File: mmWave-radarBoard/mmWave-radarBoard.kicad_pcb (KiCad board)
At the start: 6 copper layers, 100 x 100 mm, 276 parts, among them J101 Conn_01x03_Socket, J102 Conn_01x07_Socket, J103 Conn_01x06_Socket, J201 Conn_01x02_Socket, J203 USB4120-03-C, J401 Conn_01x03_Socket, J402 Conn_01x03_Socket, J403 Conn_01x03_Socket, J501 Conn_02x06_Odd_Even, Q201 BSS123, SW601 SW_DPST, SW602 SW_DPST, SW603 SW_SPDT, SW604 SW_DIP_x04, U201 TPS628502DRLR, U202 USBLC6-2P6, U203 TPS628502DRLR, U204 TPS2116DRL, U205 XI6432BRQAAMY, U206 TLV75533PDRV, U301 FT4232HQ, U302 93LCxxB, U401 TCAN1042HGVDRQ1, U402 TLIN1039DDFRQ1, U403 TRS3221EIDBR, U501 MX25R1635FZUIH0, U601 TS3A5018RSVR, U602 SN74LVC1G11DSFR, Y301 12MHz, Y501 40MHz

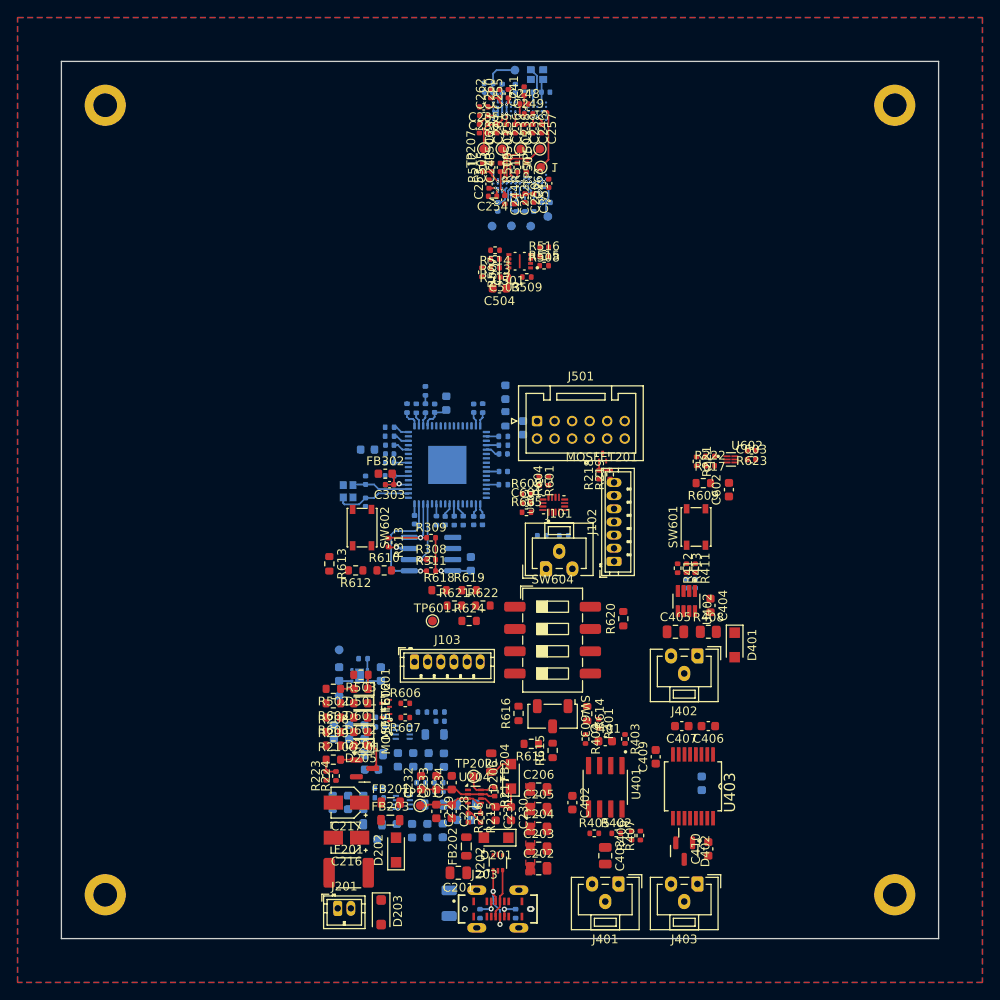
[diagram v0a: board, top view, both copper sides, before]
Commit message: Updated PCB
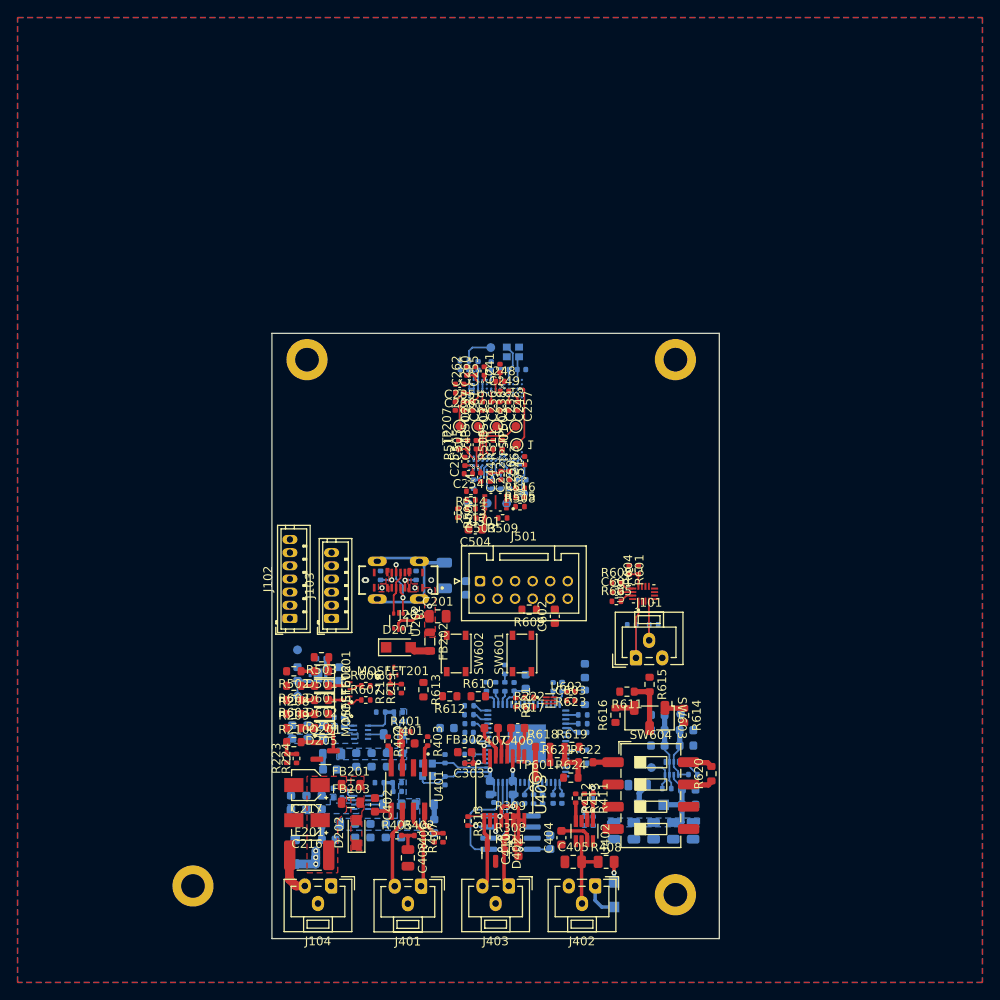
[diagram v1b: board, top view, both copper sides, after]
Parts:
- removed J201: Conn_01x02_Socket, Connector_JST:JST_ZH_B2B-ZR_1x02_P1.50mm_Vertical
- added J104: Conn_01x03_Socket, Connector_JST:JST_ZE_B03B-ZESK-D_1x03_P1.50mm_Vertical, F.Cu at (125.8, 144.0)
- C202, C203, C204, C205, C206, C228, C229, C230, C231, C232, C233, C234, C409, D203, D206, D401, FB204, R215, R216, R217, TP201, TP202, U204: moved to B.Cu
- moved R203 41.5 mm to (131.4, 108.6), turned to 90 degrees
- moved R204 39.2 mm to (135.4, 108.6), turned to 90 degrees
- moved J203 39.2 mm to (133.4, 109.1), turned to 180 degrees
- moved H102 38.3 mm to (165.0, 84.0)
- moved J102 37.5 mm to (121.0, 113.5)
- moved R207 37.4 mm to (138.7, 108.6)
- moved H101 37.0 mm to (123.0, 84.0)
- moved R617 34.3 mm to (148.3, 122.5)
- moved R623 34.3 mm to (153.1, 121.8)
- moved R221 34.3 mm to (146.8, 123.1)
- moved R222 34.3 mm to (148.3, 123.6)
- moved C603 34.3 mm to (153.1, 122.9)
- moved U602 34.3 mm to (150.7, 122.8)
- moved MOSFET201 34.1 mm to (132.9, 119.5)
- moved R218 34.1 mm to (132.5, 121.5)
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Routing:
- net Net-(J203-SHIELD-PadS1): track 0.00 -> 17.9 mm
- net VCC_3V3: track 3.19 -> 18.6 mm, vias 0 -> 1
- net /I2C_SCL: track 0.00 -> 10.4 mm
- net /COM busses/CAN_L: track 0.00 -> 9.13 mm
- net /COM busses/CAN_H: track 0.00 -> 9.13 mm
- net /COM busses/LIN: track 0.00 -> 9.01 mm
- net /COM busses/TX: track 0.00 -> 7.89 mm
- net /COM busses/RX: track 0.00 -> 7.87 mm
- net 5V_IN: track 10.3 -> 17.7 mm
- net /I2C_SDA: track 0.00 -> 6.25 mm
- net Net-(SW603-B): track 0.00 -> 5.90 mm
- net /Power/1V8_FB: track 0.00 -> 5.42 mm
- net /Power/1V2_FB: track 0.00 -> 5.17 mm
- net Net-(R619-Pad1): track 0.00 -> 5.13 mm
- net Net-(J104-Pin_3): track 0.00 -> 4.79 mm
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- added copper zone on B.Cu, net 5V_IN
- added copper zone on B.Cu, net 5V_IN_USB
- added copper zone on F.Cu, net DC_IN
- added copper zone on F.Cu, net Net-(D202-A)
- added copper zone on B.Cu, net REG_OUT_1V2
- added copper zone on B.Cu, net REG_OUT_1V8
- added copper zone on F.Cu, net USB_5V
- added copper zone on In2.Cu, net USB_5V
- removed copper zone on F.Cu, net 5V_IN_USB
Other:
- board size 100 x 100 mm -> 51 x 69 mm

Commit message: Updated schematic and layout PCB
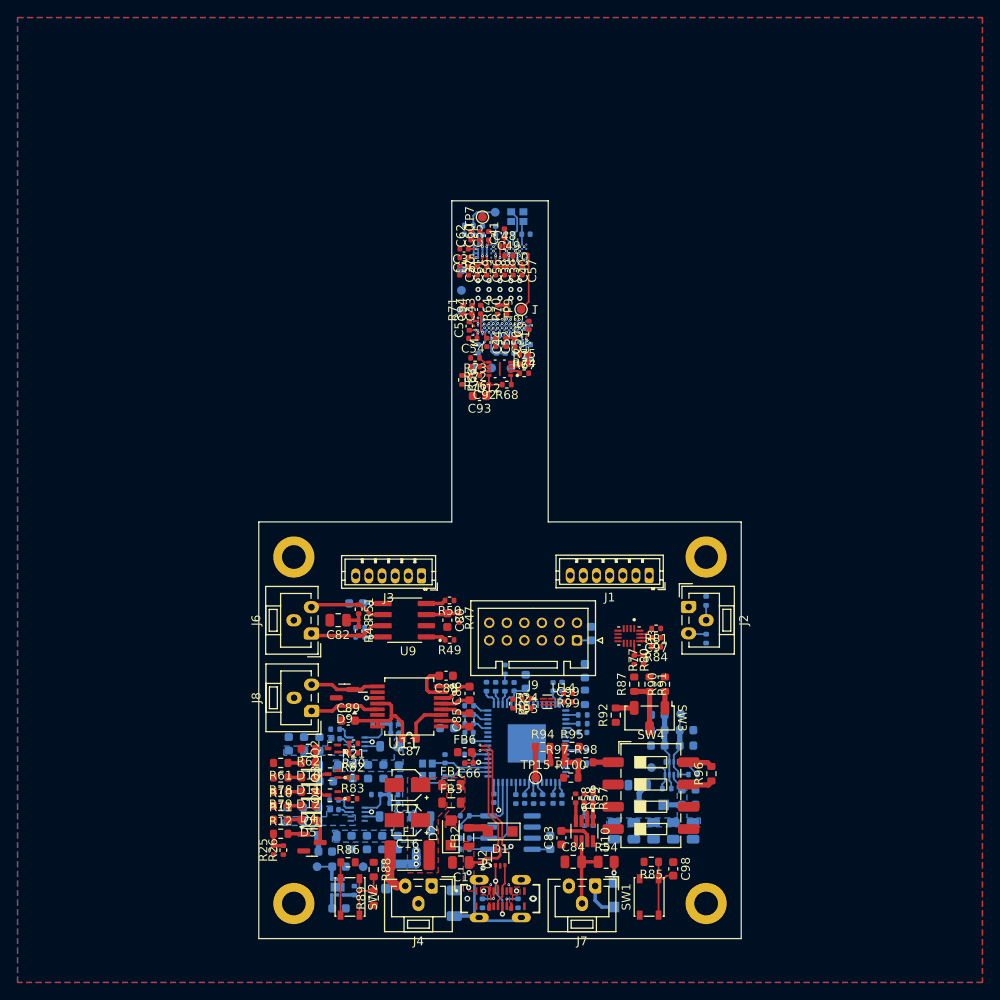
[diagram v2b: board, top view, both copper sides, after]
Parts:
- C81: renamed from C402; moved to B.Cu
- C87: renamed from C408; moved to F.Cu
- C88: renamed from C409; moved to F.Cu
- Q2: renamed from MOSFET201; footprint SSM3K35AMFV:VESM_TOS-L -> SSM3K35AMFV:VESM_TOS-M
- Q3: renamed from MOSFET601; footprint SSM3K35AMFV:VESM_TOS-L -> SSM3K35AMFV:VESM_TOS-M
- Q4: renamed from MOSFET602; footprint SSM3K35AMFV:VESM_TOS-L -> SSM3K35AMFV:VESM_TOS-M
- R35: renamed from R308; moved to B.Cu
- R36: renamed from R309; moved to B.Cu
- R38: renamed from R311; moved to B.Cu
- R40: renamed from R313; moved to B.Cu
- R52: renamed from R406; moved to B.Cu
- R53: renamed from R407; moved to B.Cu
- TP11: renamed from TP503; moved to B.Cu
- TP13: renamed from TP505; moved to B.Cu
- TP14: renamed from TP506; moved to B.Cu
- moved J1 41.2 mm to (162.0, 108.6), turned to 180 degrees
- moved R5 40.5 mm to (147.1, 146.0), turned to -90 degrees
- moved R6 38.1 mm to (143.0, 146.0), turned to -90 degrees
- moved J5 38.1 mm to (145.0, 145.4), turned to 0 degrees
- moved R9 37.4 mm to (139.8, 146.0), turned to 90 degrees
- moved R85 31.9 mm to (162.2, 141.2)
- moved C98 31.8 mm to (164.8, 142.1), turned to -90 degrees
- moved J6 31.4 mm to (123.5, 115.2), turned to 90 degrees
- moved SW1 31.3 mm to (162.0, 145.2)
- moved SW2 30.3 mm to (127.9, 145.2)
- moved J8 30.1 mm to (123.5, 124.0), turned to 90 degrees
- moved U2 29.4 mm to (145.0, 140.8), turned to 90 degrees
- moved C82 28.2 mm to (126.5, 113.7), turned to 180 degrees
- moved C1 28.2 mm to (140.5, 141.3), turned to 180 degrees
- moved C46 26.7 mm to (126.7, 146.6), turned to 0 degrees
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- renumbered C201 to C1, C210 to C10, C211 to C11, C212 to C12, C213 to C13, C214 to C14, C215 to C15, C216 to C16, C217 to C17, C218 to C18, C219 to C19, C202 to C2, C220 to C20, C221 to C21, C222 to C22, C223 to C23, C224 to C24, C225 to C25, C226 to C26, C227 to C27, C228 to C28, C229 to C29, C203 to C3, C230 to C30, C231 to C31, C232 to C32, C233 to C33, C234 to C34, C235 to C35, C236 to C36, C237 to C37, C238 to C38, C239 to C39, C204 to C4, C240 to C40, C241 to C41, C242 to C42, C243 to C43, C244 to C44, C245 to C45, C246 to C46, C247 to C47, C248 to C48, C249 to C49, C205 to C5, C250 to C50, C251 to C51, C252 to C52, C253 to C53, C254 to C54, C255 to C55, C256 to C56, C257 to C57, C258 to C58, C259 to C59, C206 to C6, C260 to C60, C261 to C61, C262 to C62, C263 to C63, C301 to C64, C302 to C65, C303 to C66, C304 to C67, C305 to C68, C306 to C69, C207 to C7, C307 to C70, C308 to C71, C309 to C72, C310 to C73, C311 to C74, C312 to C75, C313 to C76, C314 to C77, C315 to C78, C316 to C79, C208 to C8, C401 to C80, C403 to C82, C404 to C83, C405 to C84, C406 to C85, C407 to C86, C410 to C89, C209 to C9, C501 to C90, C502 to C91, C503 to C92, C504 to C93, C505 to C94, C506 to C95, C507 to C96, C601 to C97, C602 to C98, C603 to C99, D201 to D1, D501 to D10, D601 to D11, D602 to D12, D202 to D2, D203 to D3, D204 to D4, D205 to D5, D206 to D6, D301 to D7, D401 to D8, D402 to D9, F201 to F1, FB201 to FB1, FB202 to FB2, FB203 to FB3, FB204 to FB4, FB301 to FB5, FB302 to FB6, FB303 to FB7, H101 to H1, H102 to H2, H103 to H3, H104 to H4, J102 to J1, J101 to J2, J103 to J3, J104 to J4, J203 to J5, J401 to J6, J402 to J7, J403 to J8, J501 to J9, L201 to L1, L202 to L2, L203 to L3, L204 to L4, L205 to L5, Q201 to Q1, R320 to R1, R208 to R10, R624 to R100, R209 to R11, R210 to R12, R211 to R13, R212 to R14, R213 to R15, R214 to R16, R215 to R17, R216 to R18, R217 to R19, R321 to R2, R218 to R20, R219 to R21, R220 to R22, R221 to R23, R222 to R24, R223 to R25, R224 to R26, R225 to R27, R301 to R28, R302 to R29, R201 to R3, R303 to R30, R304 to R31, R305 to R32, R306 to R33, R307 to R34, R310 to R37, R312 to R39, R202 to R4, R314 to R41, R315 to R42, R316 to R43, R317 to R44, R318 to R45, R319 to R46, R401 to R47, R402 to R48, R403 to R49, R203 to R5, R404 to R50, R405 to R51, R408 to R54, R409 to R55, R410 to R56, R411 to R57, R412 to R58, R413 to R59, R204 to R6, R501 to R60, R502 to R61, R503 to R62, R504 to R63, R505 to R64, R506 to R65, R507 to R66, R508 to R67, R509 to R68, R510 to R69, R205 to R7, R511 to R70, R512 to R71, R513 to R72, R514 to R73, R515 to R74, R516 to R75, R517 to R76, R601 to R77, R602 to R78, R603 to R79, R206 to R8, R604 to R80, R605 to R81, R606 to R82, R607 to R83, R608 to R84, R609 to R85, R610 to R86, R611 to R87, R612 to R88, R613 to R89, R207 to R9, R614 to R90, R615 to R91, R616 to R92, R617 to R93, R618 to R94, R619 to R95, R620 to R96, R621 to R97, R622 to R98, R623 to R99, SW601 to SW1, SW602 to SW2, SW603 to SW3, SW604 to SW4, TP201 to TP1, TP502 to TP10, TP504 to TP12, TP601 to TP15, TP202 to TP2, TP203 to TP3, TP204 to TP4, TP205 to TP5, TP206 to TP6, TP207 to TP7, TP208 to TP8, TP501 to TP9, U201 to U1, U402 to U10, U403 to U11, U501 to U12, U601 to U13, U602 to U14, U202 to U2, U203 to U3, U204 to U4, U205 to U5, U206 to U6, U301 to U7, U302 to U8, U401 to U9, Y301 to Y1, Y501 to Y2
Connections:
- J2 pad 1: /I2C_SCL -> GND
- J2 pad 3: GND -> /I2C_SCL
- R86 pad 1: Net-(R610-Pad1) -> Net-(R86-Pad1)
- R88 pad 2: Net-(R612-Pad2) -> Net-(R88-Pad2)
- R89 pad 2: Net-(R612-Pad2) -> Net-(R88-Pad2)
- SW2 pad 1: Net-(R610-Pad1) -> Net-(R88-Pad2)
- SW2 pad 2: Net-(R612-Pad2) -> Net-(R86-Pad1)
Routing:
- net /USB_D-: track 0.00 -> 14.5 mm, vias 0 -> 1
- net /USB_D+: track 0.00 -> 13.7 mm, vias 0 -> 1
- net /I2C_SCL: track 10.4 -> 2.04 mm
- net /RADAR_~{RST}_2: track 0.00 -> 7.89 mm
- net Net-(R88-Pad2): track 0.00 -> 7.38 mm
- net RADAR_1V8: track 19.7 -> 26.2 mm
- net GND: track 0.00 -> 6.04 mm, vias 1 -> 43
- net Net-(R86-Pad1): track 0.00 -> 6.00 mm
- net /xWRL6432AOP interface/~{ERROR}_LED_WD_TP: track 7.95 -> 1.97 mm
- net FTDI_3V3: track 17.6 -> 11.7 mm, vias 1 -> 0
- net /xWRL6432AOP interface/HOST_CLK: track 5.23 -> 0.28 mm
- net /I2C_SDA: track 6.25 -> 1.69 mm
- net RADAR_3V3: track 9.16 -> 13.0 mm
- net 5V_IN_USB: track 8.18 -> 4.40 mm
- net /xWRL6432AOP interface/RTC_CLK: track 3.67 -> 0.28 mm
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- added copper zone on In1.Cu, net GND
- added copper zone on In4.Cu, net GND
- removed copper zone on In2.Cu, net GND
- removed copper zone on In3.Cu, net GND
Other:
- board size 51 x 69 mm -> 55 x 84.1 mm
